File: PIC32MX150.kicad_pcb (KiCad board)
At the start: 2 copper layers, 28 parts, among them J1 GPIO_1, J2 USB_B_Micro, J3 Barrel_Jack, J4 ICSP, J5 GPIO_2, SW1 RST, SW2 SW_SPDT, U1 PIC32MX150F128D-IPT, U2 LM22676MR-ADJ, U3 CH340C

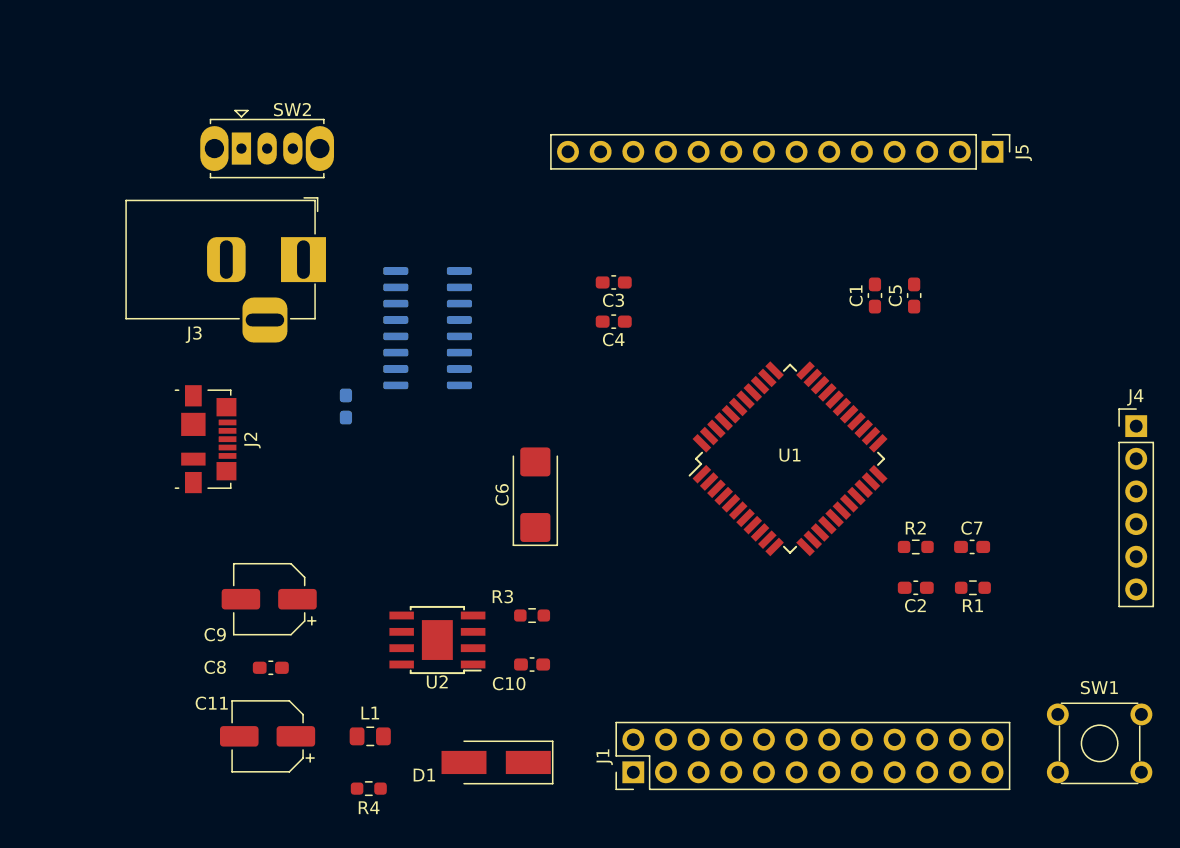
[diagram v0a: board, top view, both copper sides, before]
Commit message: LO
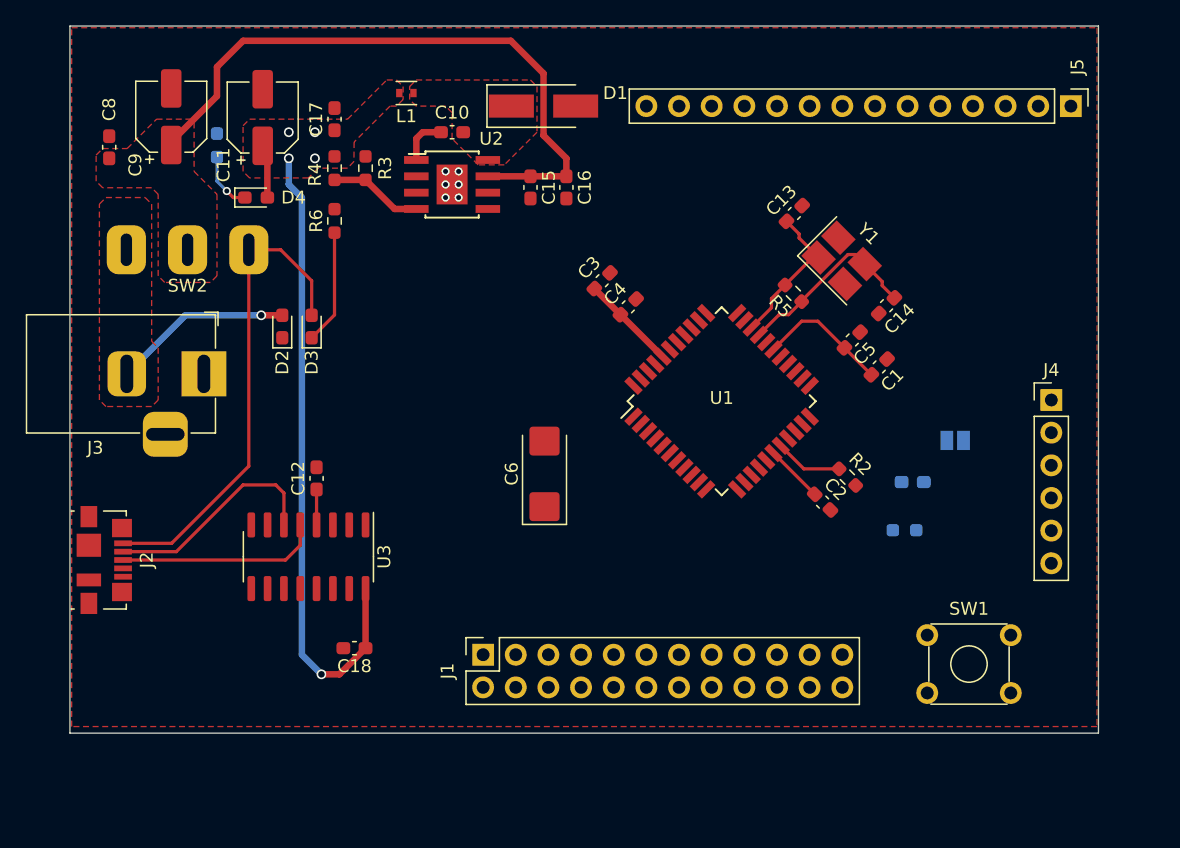
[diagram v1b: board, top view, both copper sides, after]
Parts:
- added C13: 10p, Capacitor_SMD:C_0603_1608Metric_Pad1.08x0.95mm_HandSolder, F.Cu at (96.3, 54.6)
- added C14: 10p, Capacitor_SMD:C_0603_1608Metric_Pad1.08x0.95mm_HandSolder, F.Cu at (103.5, 61.8)
- added C15: 1u, Capacitor_SMD:C_0603_1608Metric_Pad1.08x0.95mm_HandSolder, F.Cu at (75.8, 52.6)
- added C16: 100n, Capacitor_SMD:C_0603_1608Metric_Pad1.08x0.95mm_HandSolder, F.Cu at (78.6, 52.6)
- added C17: 100n, Capacitor_SMD:C_0603_1608Metric_Pad1.08x0.95mm_HandSolder, F.Cu at (60.6, 47.2)
- added C18: 100n, Capacitor_SMD:C_0603_1608Metric_Pad1.08x0.95mm_HandSolder, F.Cu at (62.1, 88.4)
- added D2: LED_B, LED_SMD:LED_0603_1608Metric_Pad1.05x0.95mm_HandSolder, F.Cu at (56.5, 63.4)
- added D3: LED_B, LED_SMD:LED_0603_1608Metric_Pad1.05x0.95mm_HandSolder, F.Cu at (58.8, 63.4)
- added D4: LED_G, LED_SMD:LED_0603_1608Metric_Pad1.05x0.95mm_HandSolder, F.Cu at (54.5, 53.3)
- added JP1: Jumper_NO_Small, Jumper:SolderJumper-2_P1.3mm_Open_Pad1.0x1.5mm, B.Cu at (108.9, 72.2)
- added R5: 1M, Resistor_SMD:R_0603_1608Metric_Pad0.98x0.95mm_HandSolder, F.Cu at (96.3, 60.8)
- added R6: 1.5K, Resistor_SMD:R_0603_1608Metric_Pad0.98x0.95mm_HandSolder, F.Cu at (60.6, 55.2)
- added R7: 1K, Resistor_SMD:R_0603_1608Metric_Pad0.98x0.95mm_HandSolder, B.Cu at (51.4, 49.3)
- added Y1: TSX3225, Crystal:Crystal_SMD_SeikoEpson_TSX3225-4Pin_3.2x2.5mm_HandSoldering, F.Cu at (100.0, 58.3)
- C12, U3: moved to F.Cu
- C7, R1: moved to B.Cu
- J1: footprint Connector_PinHeader_2.54mm:PinHeader_2x12_P2.54mm_Vertical -> Connector_PinSocket_2.54mm:PinSocket_2x12_P2.54mm_Vertical
- L1: footprint Inductor_SMD:L_0805_2012Metric_Pad1.15x1.40mm_HandSolder -> Inductor_SMD:L_Taiyo-Yuden_MD-1616
- SW2: footprint Button_Switch_THT:SW_Slide_1P2T_CK_OS102011MS2Q -> Custom_Libs:SPDT_SW_Big
- moved D1 51.2 mm to (76.8, 46.2), turned to 0 degrees
- moved L1 50.1 mm to (66.2, 45.2)
- moved R4 48.3 mm to (60.6, 51.1), turned to 270 degrees
- moved C11 48.1 mm to (55.0, 47.1), turned to 90 degrees
- moved C8 42.4 mm to (43.1, 49.4), turned to 90 degrees
- moved C10 41.9 mm to (69.7, 48.3)
- moved C9 38.3 mm to (47.9, 47.1), turned to 90 degrees
- moved R3 37.1 mm to (63.0, 51.1), turned to 90 degrees
- moved U2 35.5 mm to (69.7, 52.3), turned to 0 degrees
- moved U3 20.1 mm to (58.5, 81.3), turned to 270 degrees
- moved J1 14.8 mm to (72.1, 88.9)
- moved J2 12.4 mm to (42.7, 81.5)
- moved SW1 11.9 mm to (106.7, 87.4)
- moved J3 11.8 mm to (50.4, 67.1)
- moved C2 9.85 mm to (98.5, 77.0), turned to 315 degrees
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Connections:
- R1 pad 2: Net-(C7-Pad1) -> Net-(JP1-Pad1)
- R2 pad 2: Net-(C7-Pad1) -> Net-(JP1-Pad1)
- U1 pad 30: (no net) -> /OSC1
- U1 pad 31: (no net) -> /OSC2
- U2 pad 5: (no net) -> GND
- U3 pad 16: +5V -> +3V3
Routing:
- net +3V3: track 0.00 -> 76.6 mm, vias 0 -> 5
- net +5V: track 0.00 -> 49.7 mm
- net /PWR_USB: track 0.00 -> 37.7 mm
- net Net-(J2-Pad2): track 0.00 -> 17.4 mm
- net Net-(J2-Pad3): track 0.00 -> 15.8 mm
- net /OSC1: track 0.00 -> 14.7 mm
- net /PWR_DC: track 0.00 -> 14.0 mm, vias 0 -> 1
- net /OSC2: track 0.00 -> 12.3 mm
- net Net-(D2-Pad1): track 0.00 -> 8.91 mm
- net Net-(R3-Pad1): track 0.00 -> 7.32 mm
- net /MCLR: track 0.00 -> 5.28 mm
- net Net-(D4-Pad1): track 0.00 -> 4.58 mm, vias 0 -> 1
- net Net-(C10-Pad2): track 0.00 -> 3.79 mm
- net Net-(C12-Pad1): track 0.00 -> 2.76 mm
- net GND: vias 0 -> 6
- added copper zone on F.Cu, net +3V3
- added copper zone on F.Cu, net +5V
- added copper zone on F.Cu, net /PWR_DC
- added copper zone on F.Cu, net GND
- added copper zone on F.Cu, net Net-(C10-Pad1)
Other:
- board outline added: 80 x 55 mm
- net class Default: clearance 0.254 -> 0.2032; via_dia 0.508 -> 0.635; via_drill 0.3048 -> 0.381
- net class PWR added: clearance 0.2032, trace_width 0.508, via_dia 0.762, via_drill 0.508
- rule trace_clearance: 0.254 -> 0.2032
